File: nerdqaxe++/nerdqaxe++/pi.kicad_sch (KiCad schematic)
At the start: 20 parts, among them J5 Conn_01x12-Socket, J6 Conn_01x12-Socket, J7 Conn_01x12-Header, J8 Conn_01x12-Header, M1 Fan_4pin, M2 Fan_4pin, U30 T-Display-S3, U32 EMC2302-1, U33 TXU0102-DCU, U37 TMP1075

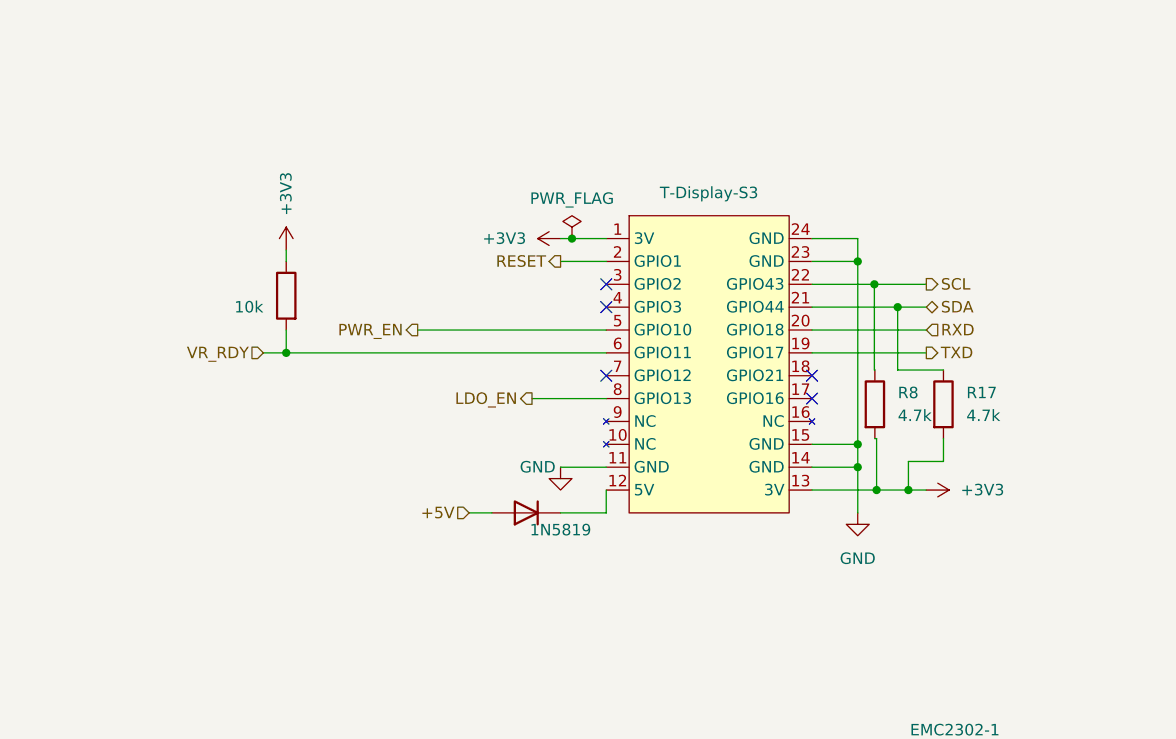
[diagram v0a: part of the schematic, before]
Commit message: feature complete
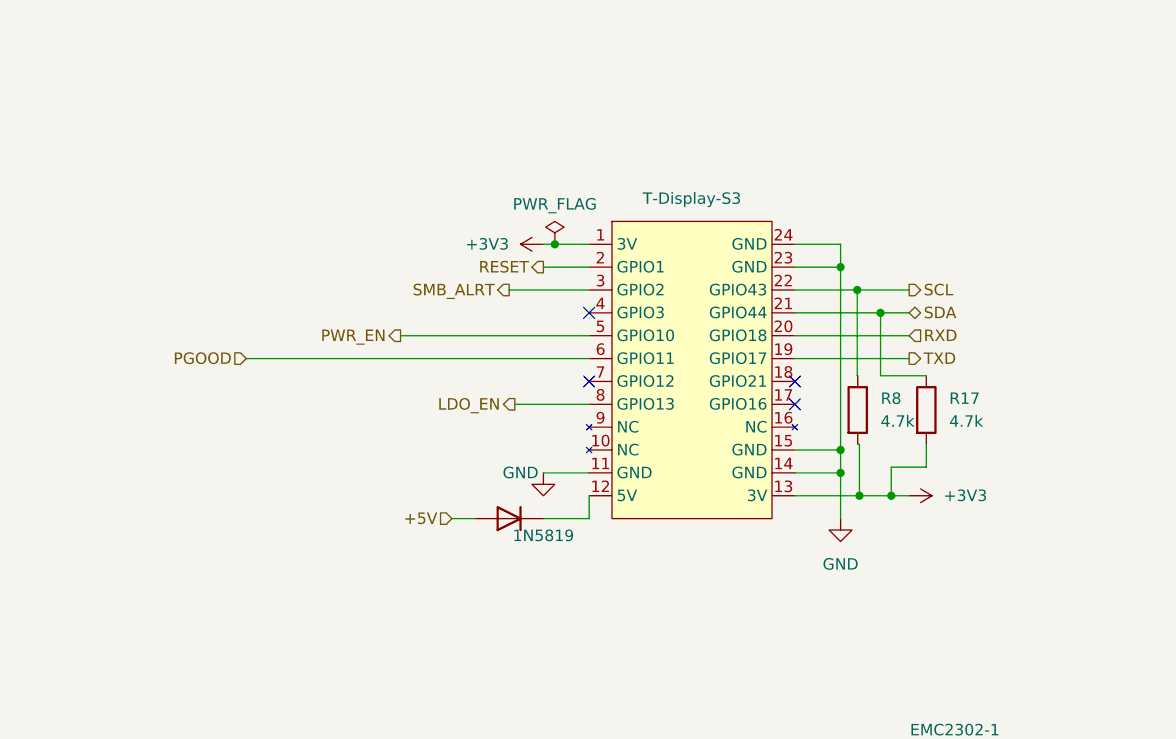
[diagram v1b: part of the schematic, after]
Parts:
- removed R36: 10k, Resistor_SMD:R_0402_1005Metric, symbol Device:R
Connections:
- net SMB_ALRT: now reaches U30.3 (GPIO2)
- net VR_RDY renamed PGOOD
- no-connect marks 8 -> 7
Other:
- moved on the sheet: R17, R8
